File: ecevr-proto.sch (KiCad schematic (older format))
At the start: 5 parts, among them U14 74LVC1G06

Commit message: further work...
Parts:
- H5, H6, H7, H8: Manufacturer (none) -> Essentra; Part (none) -> FF-13-P3.5X6.0B
- U21: renamed from U14; footprint proj_footprints:SOT-5x3 -> Package_TO_SOT_SMD:SOT-353_SC-70-5; symbol fmc:74LVC1G06 -> fmc:74LVC1G38
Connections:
- net +1V8: now also U21.5 (VCC)
- net +3V3: no longer U21.5 (VCC)
- net IO_L5P_T0_AD9P_15: no longer U21.2
- net IO_L3N_T0_DQS_AD1N_15: now reaches U21.1
- net IO_L3N_T0_DQS_AD1N_15: now also U21.2

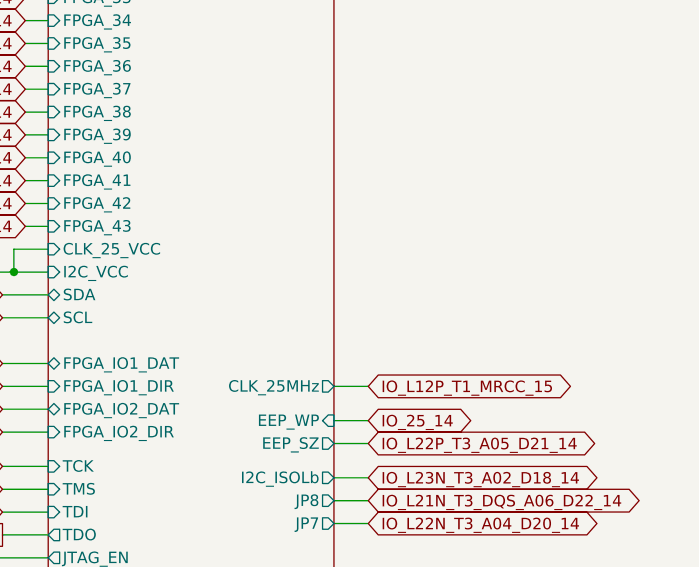
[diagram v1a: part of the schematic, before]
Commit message: added 3rd GPIO
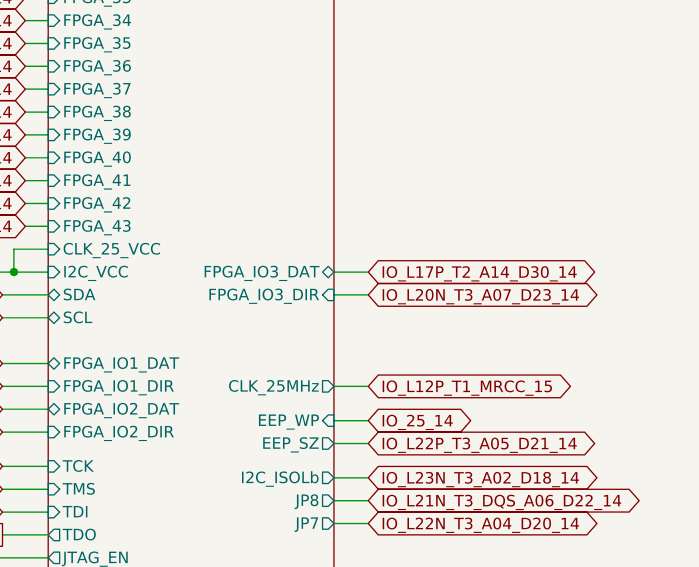
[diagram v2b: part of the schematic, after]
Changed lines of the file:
@@
 $Descr USLetter 11000 8500
 encoding utf-8
-Sheet 1 20
+Sheet 1 21
 Title ""
 Date ""
@@
 F63 "TMS" I L 7900 6150 50
 F64 "JTAG_EN" O L 7900 6450 50
+F65 "FPGA_IO3_DIR" I R 9150 5300 50
+F66 "FPGA_IO3_DAT" B R 9150 5200 50
 $EndSheet
 Text GLabel 9300 5850 2    50   BiDi ~ 0
@@
 Wire Wire Line
 	1700 7400 1700 7450
+Text GLabel 9300 5200 2    50   BiDi ~ 0
+IO_L17P_T2_A14_D30_14
+Wire Wire Line
+	9300 5200 9150 5200
+Text GLabel 9300 5300 2    50   BiDi ~ 0
+IO_L20N_T3_A07_D23_14
+Wire Wire Line
+	9300 5300 9150 5300
 $EndSCHEMATC
